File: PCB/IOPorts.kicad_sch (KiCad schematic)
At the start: 0 parts

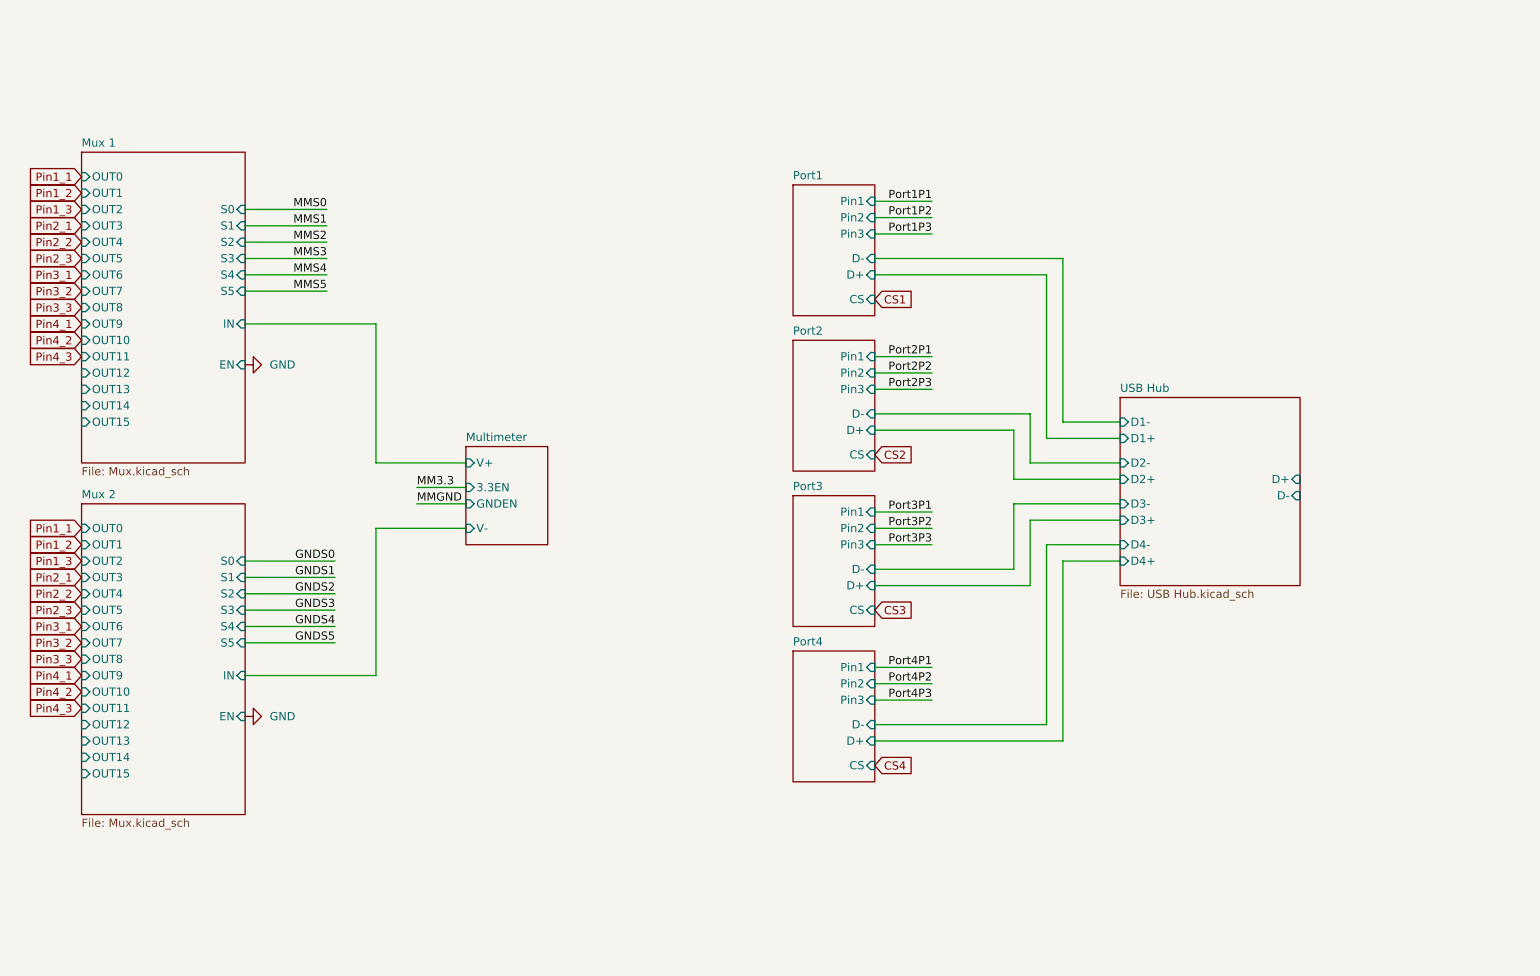
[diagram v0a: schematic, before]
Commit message: Updated PCB
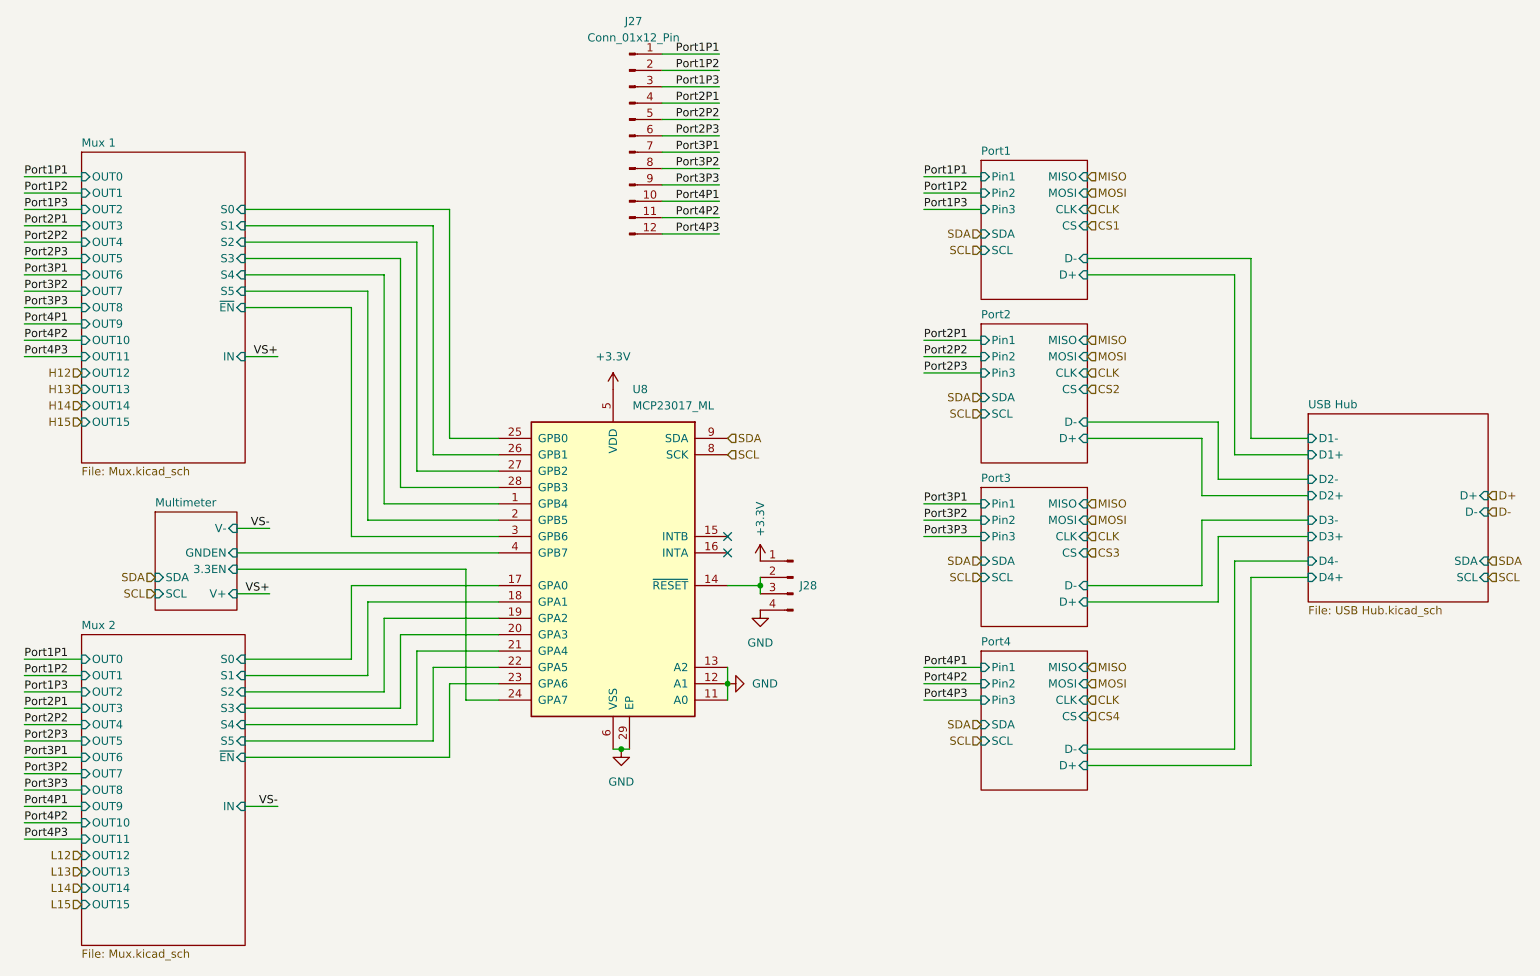
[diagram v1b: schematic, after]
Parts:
- added J27: Conn_01x12_Pin, Connector_PinHeader_1.27mm:PinHeader_1x12_P1.27mm_Vertical, symbol Connector:Conn_01x12_Pin
- added J28: Conn_01x04_Pin, Connector_PinHeader_1.27mm:PinHeader_1x04_P1.27mm_Vertical, symbol Connector:Conn_01x04_Pin
- added U8: MCP23017_ML, Package_DFN_QFN:QFN-28-1EP_6x6mm_P0.65mm_EP4.25x4.25mm, symbol Interface_Expansion:MCP23017_ML
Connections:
- net GND: now also J28.4 (Pin_4), U8.11 (A0), U8.12 (A1), U8.13 (A2), U8.29 (EP), U8.6 (VSS)
- net Port1P1: now also J27.1 (Pin_1)
- net Port1P2: now also J27.2 (Pin_2)
- net Port1P3: now also J27.3 (Pin_3)
- net Port2P1: now also J27.4 (Pin_4)
- net Port2P2: now also J27.5 (Pin_5)
- net Port2P3: now also J27.6 (Pin_6)
- net Port3P1: now also J27.7 (Pin_7)
- net Port3P2: now also J27.8 (Pin_8)
- net Port3P3: now also J27.9 (Pin_9)
- net Port4P1: now also J27.10 (Pin_10)
- net Port4P2: now also J27.11 (Pin_11)
- net Port4P3: now also J27.12 (Pin_12)
- new net: J28.2 (Pin_2), J28.3 (Pin_3), U8.14 (~{RESET})
- new net +3.3V: J28.1 (Pin_1), U8.5 (VDD)
- new net Multimeter/3.3EN: U8.24 (GPA7)
- new net Multimeter/GNDEN: U8.4 (GPB7)
- new net Mux 1/S0: U8.25 (GPB0)
- new net Mux 1/S1: U8.26 (GPB1)
- new net Mux 1/S2: U8.27 (GPB2)
- new net Mux 1/S3: U8.28 (GPB3)
- new net Mux 1/S4: U8.1 (GPB4)
- new net Mux 1/S5: U8.2 (GPB5)
- new net Mux 1/~{EN}: U8.3 (GPB6)
- new net Mux 2/S0: U8.17 (GPA0)
- new net Mux 2/S1: U8.18 (GPA1)
- new net Mux 2/S2: U8.19 (GPA2)
- new net Mux 2/S3: U8.20 (GPA3)
- new net Mux 2/S4: U8.21 (GPA4)
- new net Mux 2/S5: U8.22 (GPA5)
- new net Mux 2/~{EN}: U8.23 (GPA6)
- new net SCL: U8.8 (SCK)
- new net SDA: U8.9 (SDA)
- no-connect marks 0 -> 2
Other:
- sheet Multimeter ports: added SCL, SDA; removed none
- sheet Mux 1 ports: added ~{EN}; removed EN
- sheet Mux 2 ports: added ~{EN}; removed EN
- sheet Port1 ports: added CLK, MISO, MOSI, SCL, SDA; removed none
- sheet Port2 ports: added CLK, MISO, MOSI, SCL, SDA; removed none
- sheet Port3 ports: added CLK, MISO, MOSI, SCL, SDA; removed none
- sheet Port4 ports: added CLK, MISO, MOSI, SCL, SDA; removed none
- sheet USB Hub ports: added SCL, SDA; removed none
